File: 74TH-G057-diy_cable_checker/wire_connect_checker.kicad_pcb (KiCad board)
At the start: 2 copper layers, 53.5 x 69.5 mm, 73 parts, among them J1 USB2.0-C_SMT, Q1 2N7002, Q10 2N7002, Q2 2N7002, Q3 2N7002, Q4 2N7002, Q5 2N7002, Q6 2N7002, Q7 2N7002, Q8 2N7002, Q9 2N7002, U1 CH32V003F4P6, U3 AMS1117, U4 CH213K

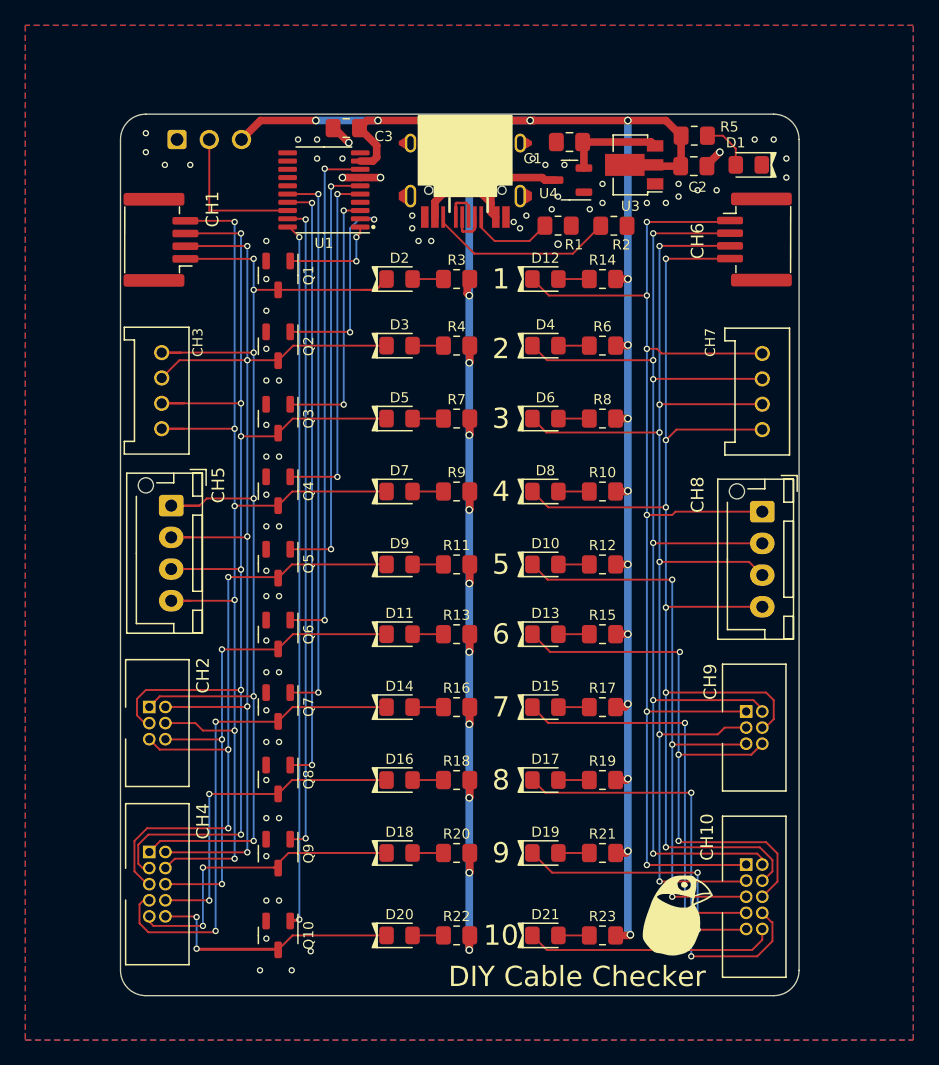
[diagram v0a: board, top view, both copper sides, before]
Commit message: cable checker
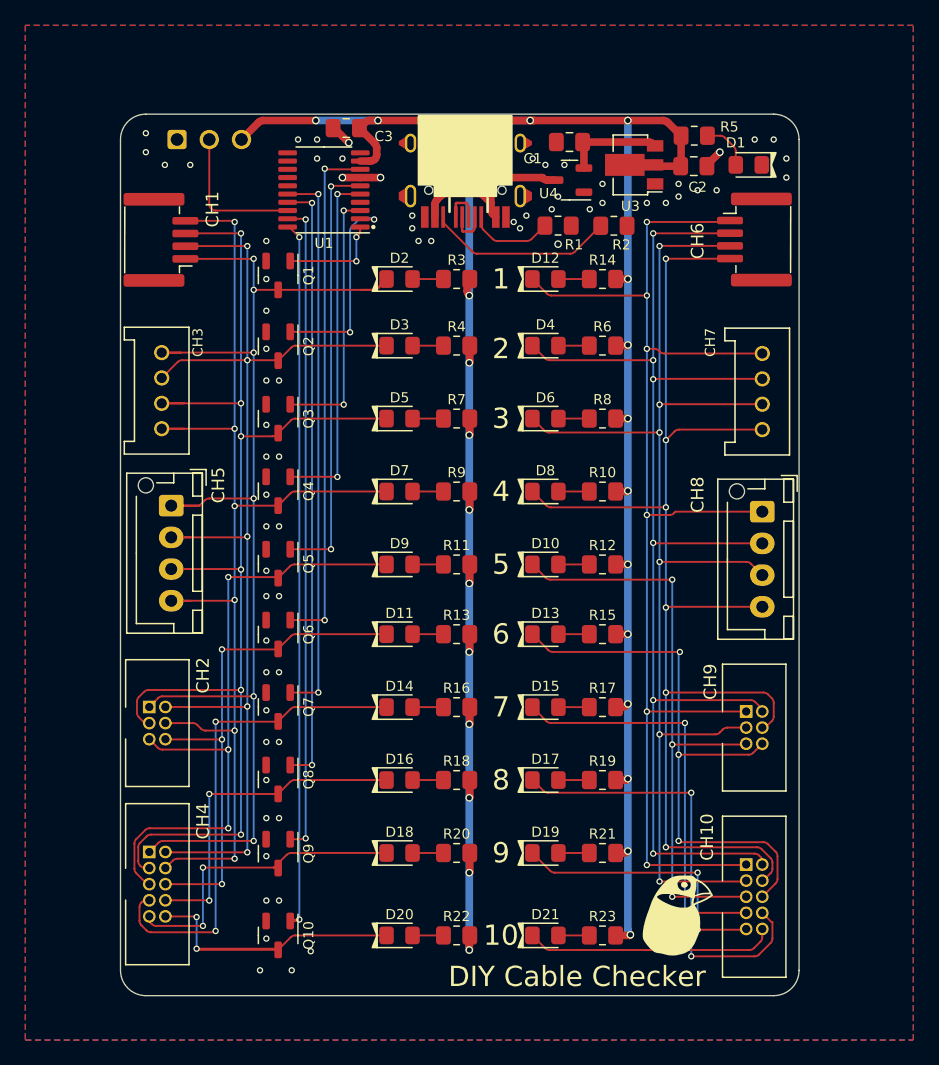
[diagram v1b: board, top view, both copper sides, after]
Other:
- board text added: "74TH-G057-${REVISION}"
- board text removed: "74TH-G057-1.0.0"
